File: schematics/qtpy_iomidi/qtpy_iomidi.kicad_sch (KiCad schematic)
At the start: 25 parts, among them J1 AudioJack4, J2 AudioJack4, J4 Conn_01x02_Pin, J5 OLED-128x64, SW1 SW_Omron_B3FS, U2 H11L1

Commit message: more pcb tweaking
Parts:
- U1: footprint todbot_eagle2023:QTPY_TH -> todbot_eagle2023:QTPY_TH_HEADERSOCKET
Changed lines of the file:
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@@
 			)
 		)
-		(property "Footprint" "todbot_eagle2023:QTPY_TH"
+		(property "Footprint" "todbot_eagle2023:QTPY_TH_HEADERSOCKET"
 			(at 95.504 53.34 0)
 			(effects

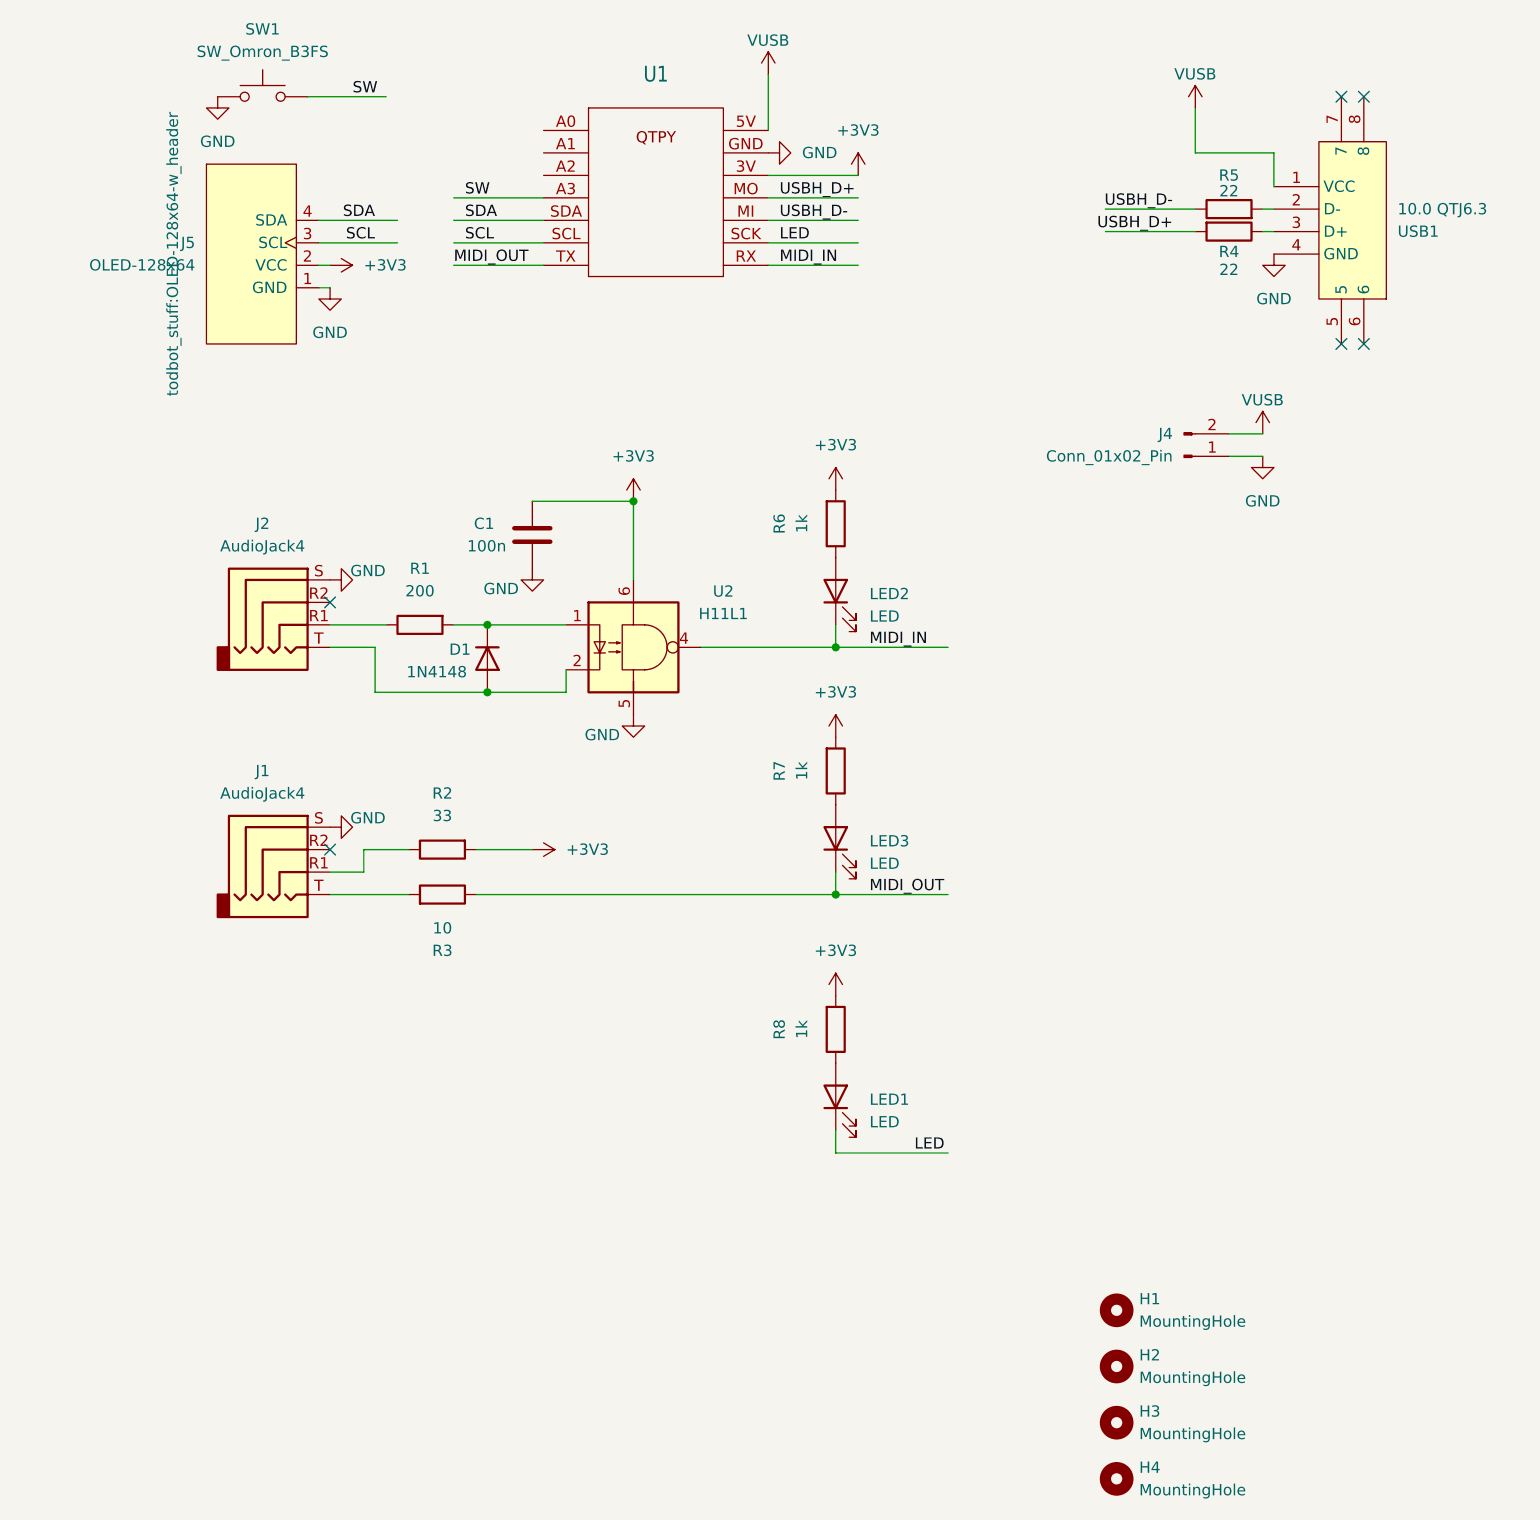
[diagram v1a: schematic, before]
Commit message: added encoder
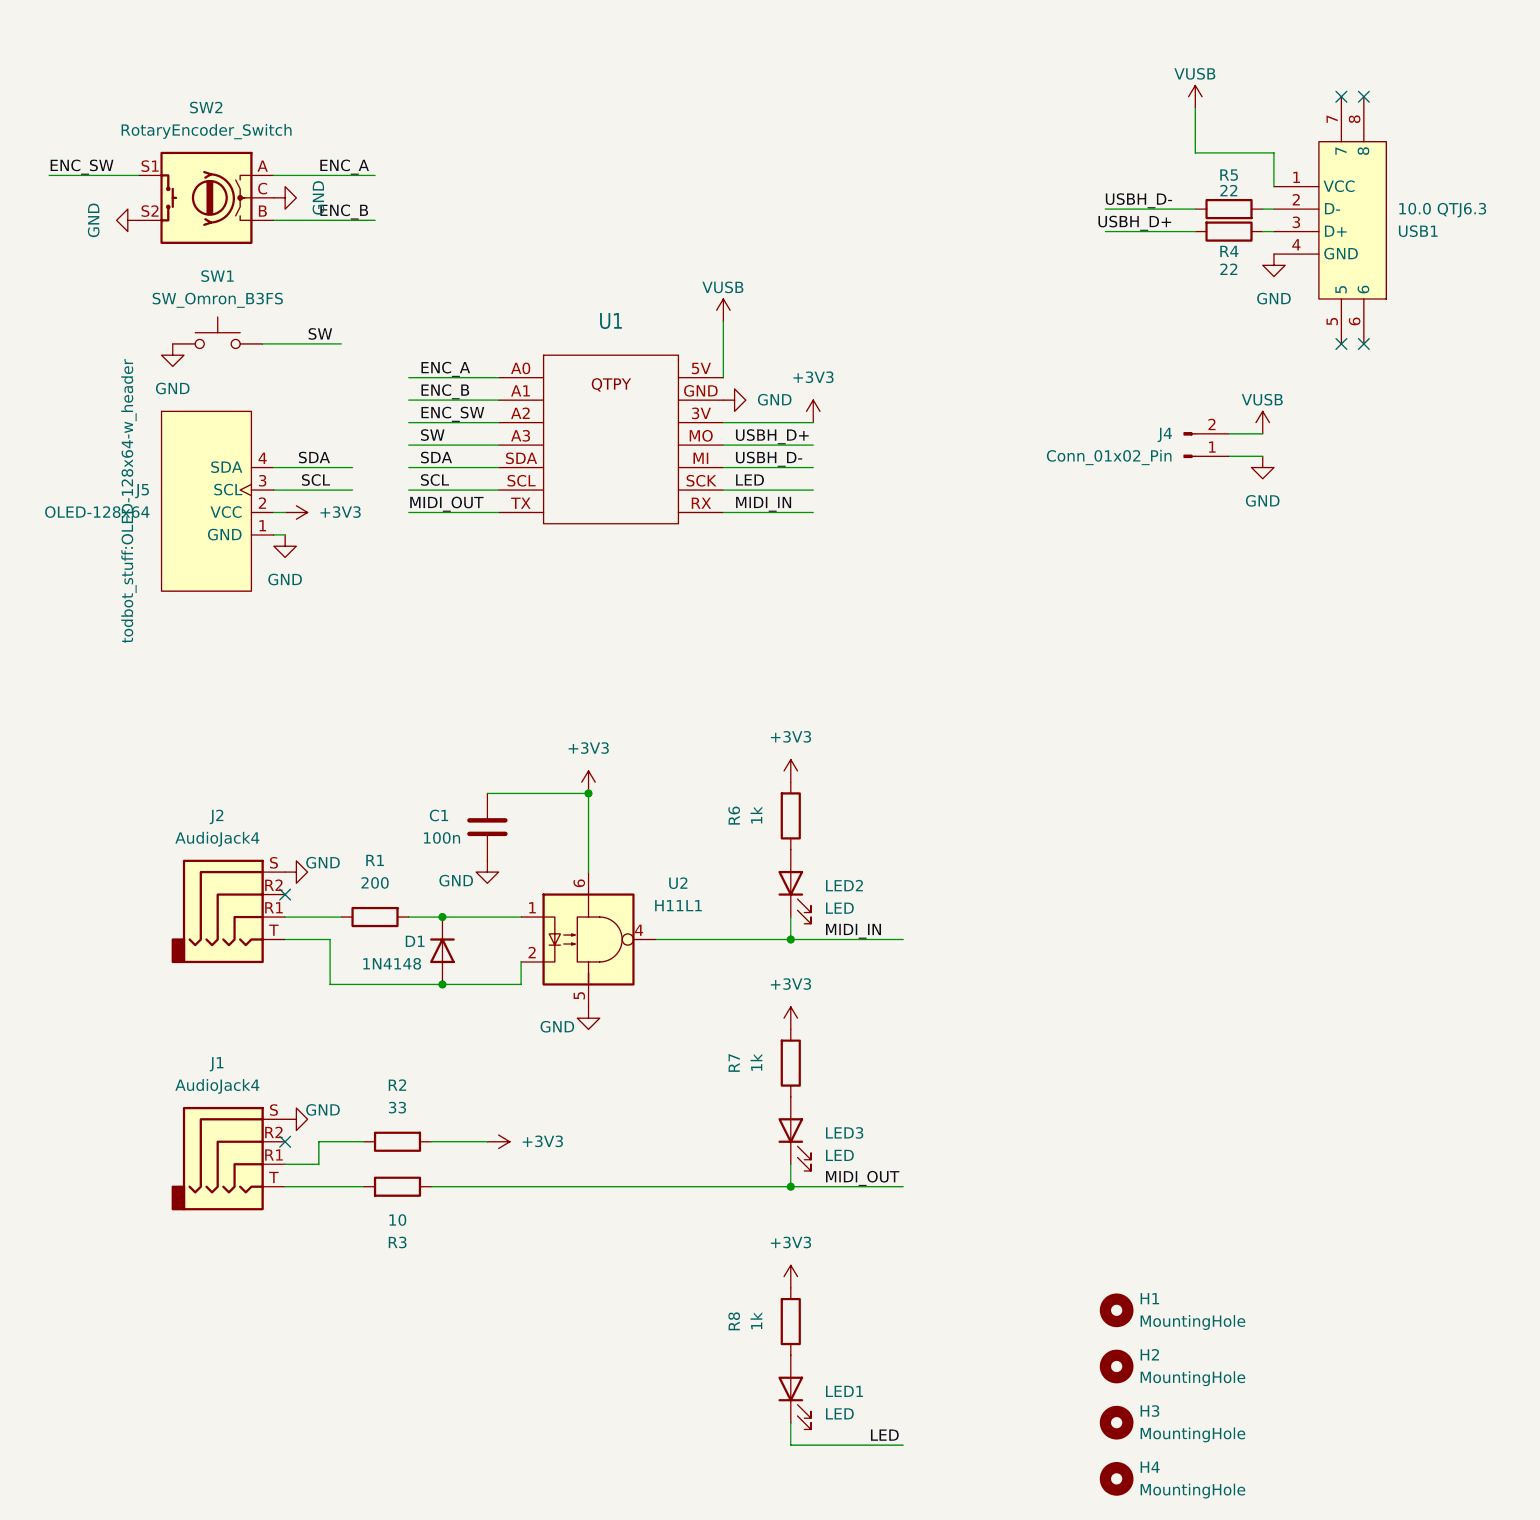
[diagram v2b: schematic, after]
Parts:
- added SW2: RotaryEncoder_Switch, Rotary_Encoder:RotaryEncoder_Alps_EC11E-Switch_Vertical_H20mm_CircularMountingHoles, symbol Device:RotaryEncoder_Switch
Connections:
- net GND: now also SW2.C, SW2.S2
- net ENC_A: now reaches U1.A0
- net ENC_A: now also SW2.A
- net ENC_B: now reaches U1.A1 (9)
- net ENC_B: now also SW2.B
- net ENC_SW: now reaches U1.A2
- net ENC_SW: now also SW2.S1
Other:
- moved on the sheet: C1, D1, J1, J2, J5, LED1, LED2, LED3, R1, R2, R3, R6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
